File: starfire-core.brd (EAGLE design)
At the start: 60 x 52 mm, 70 parts, among them Q1 FDN340P, Y1 16MHZ

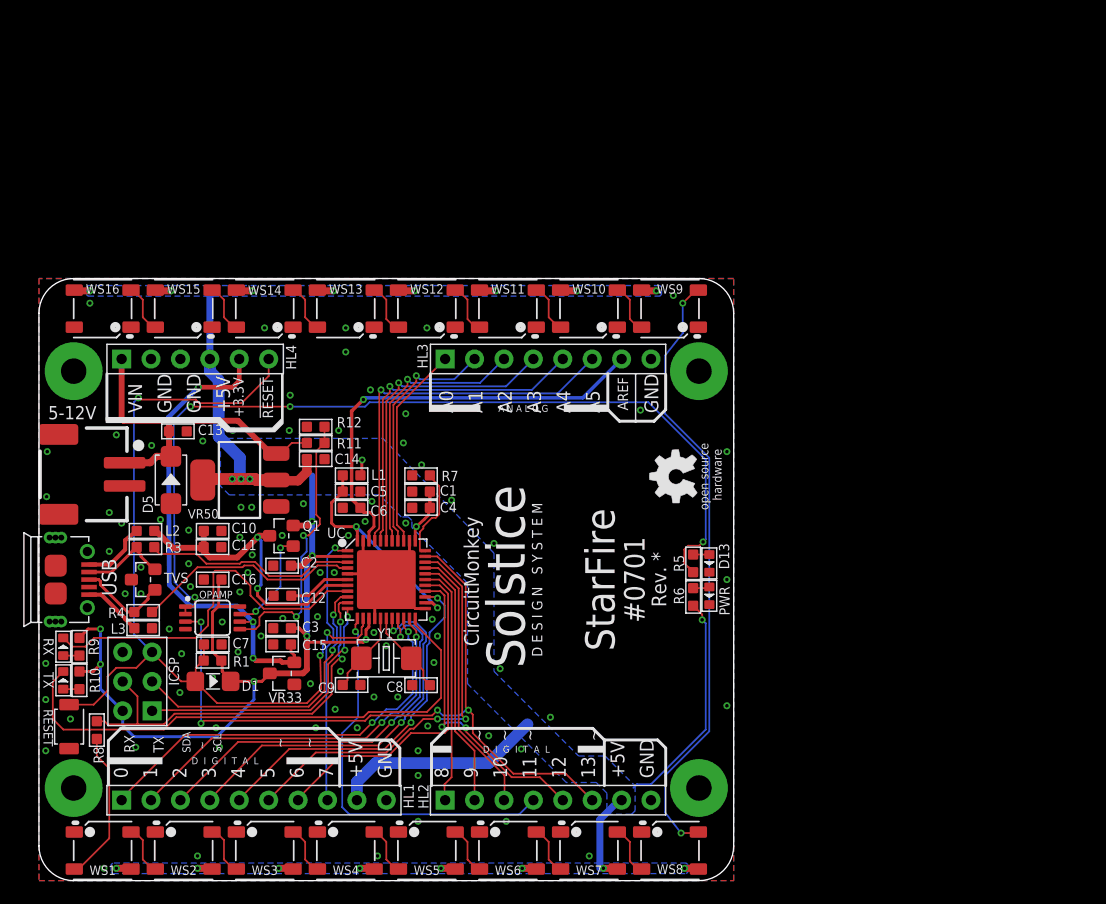
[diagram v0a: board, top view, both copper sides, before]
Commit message: Rev. A PCBs shared to world
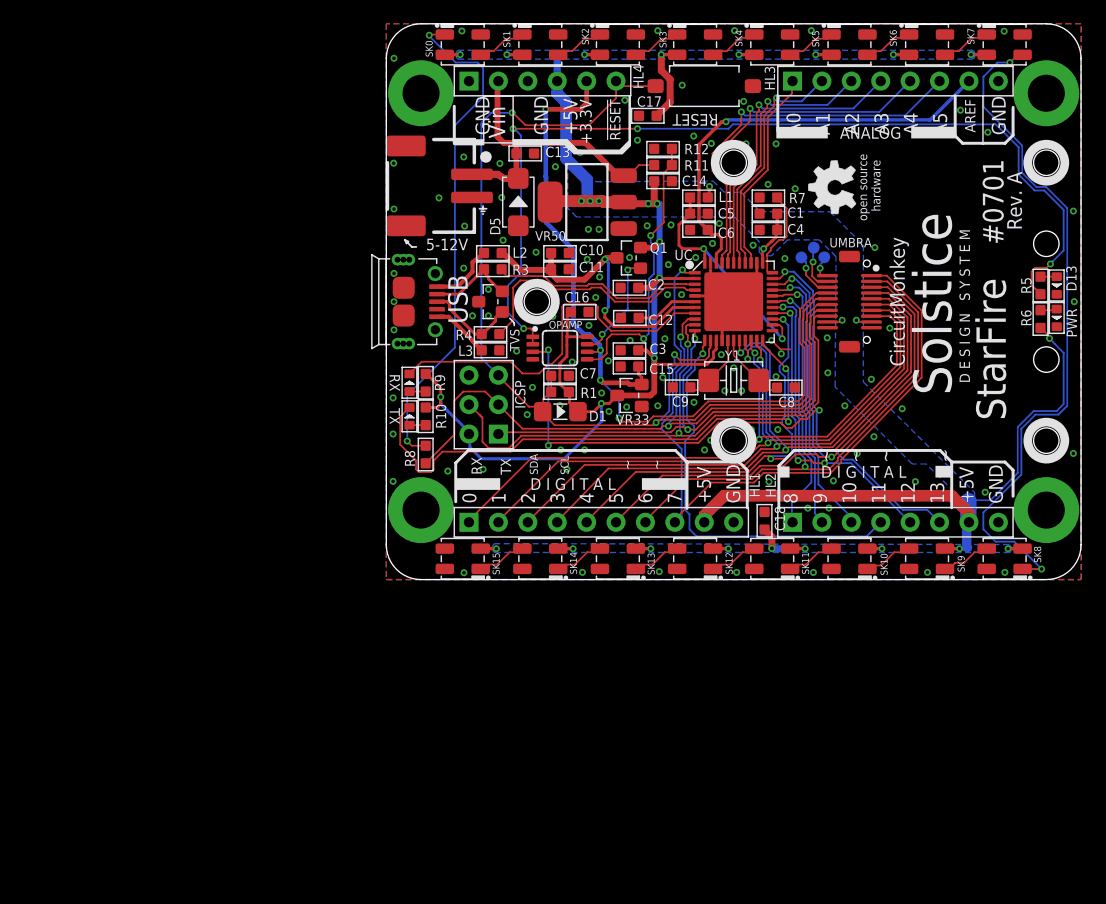
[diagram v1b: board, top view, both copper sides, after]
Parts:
- removed WS1, WS10, WS11, WS12, WS13, WS14, WS15, WS16, WS2, WS3, WS4, WS5, WS6, WS7, WS8, WS9: WS2812, led:NEOPIXEL
- added C17, C18: 10uf, Seeed-Capacitor:C0603
- added SK0, SK1, SK10, SK11, SK12, SK13, SK14, SK15, SK2, SK3, SK4, SK5, SK6, SK7, SK8, SK9: SK6812-MINI, led:SMD_3535
- added UMBRA: DF12-20DS-0.5V, co-hirose:DF12-20P-RCPT-MTL-BOSS
- added US0, US1, US2: TPSMD-040-RND, con-testpoints:SMD-040MIL-RND
- RESET: value B3U-1000P-2P-SMD -> MOM (OFF)-ON; device Seeed-Switch:SW2-2.6-3.0X2.5X1.2+0.4MM -> comp-switch:SWITCH-0635-2P-SMD
- VR33: value XC6206P332MR-G-SOT23 -> 3.3V
- moved RESET 77.9 mm to (27.5, 42.6), turned to 0 degrees
- moved C8 40.7 mm to (34.5, 16.6), turned to 90 degrees
- moved C16 39.2 mm to (16.7, 23.1), turned to 270 degrees
- moved 5-12V 39.0 mm to (0.10, 34.0)
- moved USB 38.5 mm to (1.50, 24.0)
- moved C1 38.4 mm to (33.0, 31.6)
- moved C10 38.4 mm to (15.0, 28.2)
- moved C11 38.4 mm to (15.0, 26.8)
- moved C12 38.4 mm to (21.0, 22.6)
- moved C13 38.4 mm to (12.0, 36.8)
- moved C14 38.4 mm to (23.9, 34.4)
- moved C15 38.4 mm to (21.0, 18.4)
- moved C2 38.4 mm to (21.0, 25.2)
- moved C3 38.4 mm to (21.0, 19.8)
- moved C4 38.4 mm to (33.0, 30.2)
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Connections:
- removed net MOSI/WS2812: ICSP.5, R8.1, UC.10
- removed net N$29: WS11.2, WS12.4
- removed net N$30: WS12.2, WS13.4
- removed net N$31: WS13.2, WS14.4
- removed net N$32: WS14.2, WS15.4
- removed net N$33: WS15.2, WS16.4
- removed net PIXELS: R8.2, WS1.4
- removed net SCK: ICSP.2, UC.9
- new net MOSI: ICSP.5, UC.10, UMBRA.16
- new net N$1: SK0.1, SK1.3
- new net N$12: SK6.1, SK7.3
- new net N$4: SK1.1, SK2.3
- new net N$5: SK2.1, SK3.3
- new net N$6: SK3.1, SK4.3
- new net N$9: SK4.1, SK5.3
- new net SCK/PIXELS: ICSP.2, R8.1, UC.9, UMBRA.12
- new net SL0: UMBRA.2, US0.TP
- new net SL1: UMBRA.4, US1.TP
- new net SL2: UMBRA.6, US2.TP
- net !RESET: now also RESET.1, UMBRA.10; no longer RESET.2
- net +3V3: now also UMBRA.8
- net D0: now also UMBRA.15
- net D1: now also UMBRA.13
- net D2: now also UMBRA.11
- net D3: now also UMBRA.9
- net D4: now also UMBRA.7
- net D5: now also UMBRA.5
- net D6: now also UMBRA.3
- net D7: now also UMBRA.1
- net GND: now also C17.1, C18.1, HL4.1, RESET.2, SK0.2, SK1.2, SK10.2, SK11.2, SK12.2, SK13.2, SK14.2, SK15.2, SK2.2, SK3.2, SK4.2, SK5.2, SK6.2, SK7.2, SK8.2, SK9.2, UMBRA.19, UMBRA.20; no longer HL4.2, RESET.1, WS1.3, WS10.3, WS11.3, WS12.3, WS13.3, WS14.3, WS15.3, WS16.3, WS2.3, WS3.3, WS4.3, WS5.3, WS6.3, WS7.3, WS8.3, WS9.3
- net MISO: now also UMBRA.14
- net N$11: now also SK5.1, SK6.3; no longer WS1.2, WS2.4
- net N$13: now also SK8.1, SK9.3; no longer WS2.2, WS3.4
- net N$14: now also R8.2, SK0.3; no longer WS3.2, WS4.4
- net N$15: now also SK10.3, SK9.1; no longer WS4.2, WS5.4
- net N$16: now also SK10.1, SK11.3; no longer WS5.2, WS6.4
- net N$17: now also SK11.1, SK12.3; no longer WS6.2, WS7.4
- net N$18: now also SK12.1, SK13.3; no longer WS7.2, WS8.4
- net N$19: now also SK13.1, SK14.3; no longer WS8.2, WS9.4
- net N$20: now also SK14.1, SK15.3; no longer WS10.4, WS9.2
- net N$28: now also SK7.1, SK8.3; no longer WS10.2, WS11.4
- net VCC: now also C17.2, C18.2, SK0.4, SK1.4, SK10.4, SK11.4, SK12.4, SK13.4, SK14.4, SK15.4, SK2.4, SK3.4, SK4.4, SK5.4, SK6.4, SK7.4, SK8.4, SK9.4, UMBRA.17, UMBRA.18; no longer WS1.1, WS10.1, WS11.1, WS12.1, WS13.1, WS14.1, WS15.1, WS16.1, WS2.1, WS3.1, WS4.1, WS5.1, WS6.1, WS7.1, WS8.1, WS9.1
- net VIN: now also HL4.2; no longer HL4.1
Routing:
- net SCK/PIXELS: track 0.00 -> 60.3 mm, vias 0 -> 2
- net N$28: track 4.32 -> 59.0 mm, vias 0 -> 2
- net MOSI: track 0.00 -> 54.1 mm, vias 0 -> 2
- net N$19: track 53.3 -> 4.32 mm, vias 2 -> 0
- net N$14: track 4.32 -> 43.9 mm, vias 0 -> 2
- net D7: track 23.8 -> 63.3 mm
- net MOSI/WS2812: track 35.1 -> 0.00 mm, vias 2 -> 0
- net D4: track 31.0 -> 58.5 mm
- net +3V3: track 42.0 -> 69.4 mm, vias 3 -> 4
- net D6: track 29.6 -> 55.9 mm, vias 0 -> 2
- net SCK: track 25.9 -> 0.00 mm, vias 2 -> 0
- net D5: track 35.6 -> 60.5 mm
- net D3: track 32.7 -> 57.5 mm
- net D2: track 34.5 -> 58.5 mm
- net D1: track 33.6 -> 56.5 mm
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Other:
- board size 60 x 52 mm -> 60 x 48 mm
- board text added: "Rev. A"
- board text removed: "Rev. *"
